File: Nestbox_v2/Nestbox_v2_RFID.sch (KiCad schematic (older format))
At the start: 8 parts, among them J701 RFID_CONN_01X05, Q701 Q_NMOS_DGS

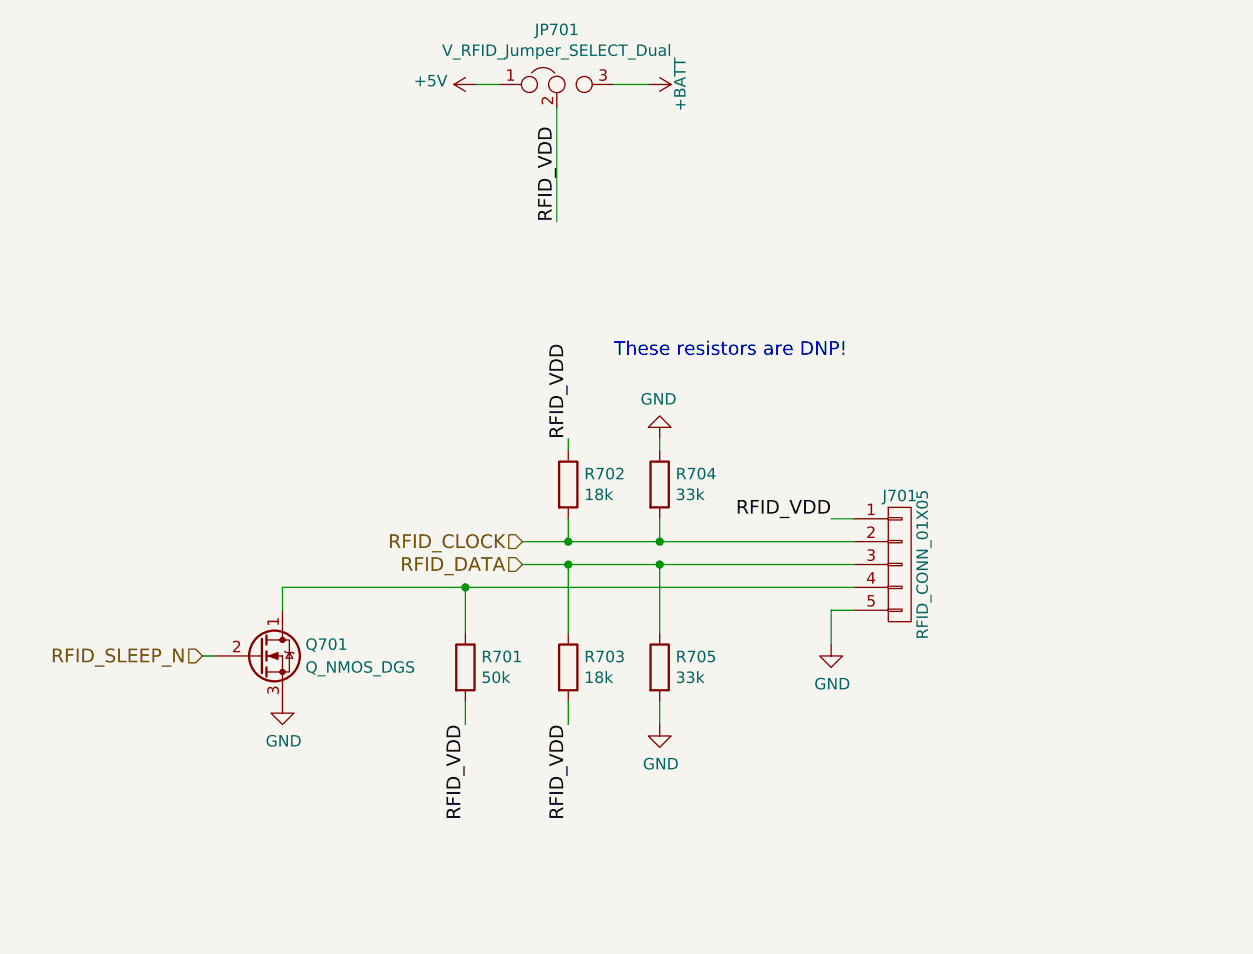
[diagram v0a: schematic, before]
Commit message: finished component placement
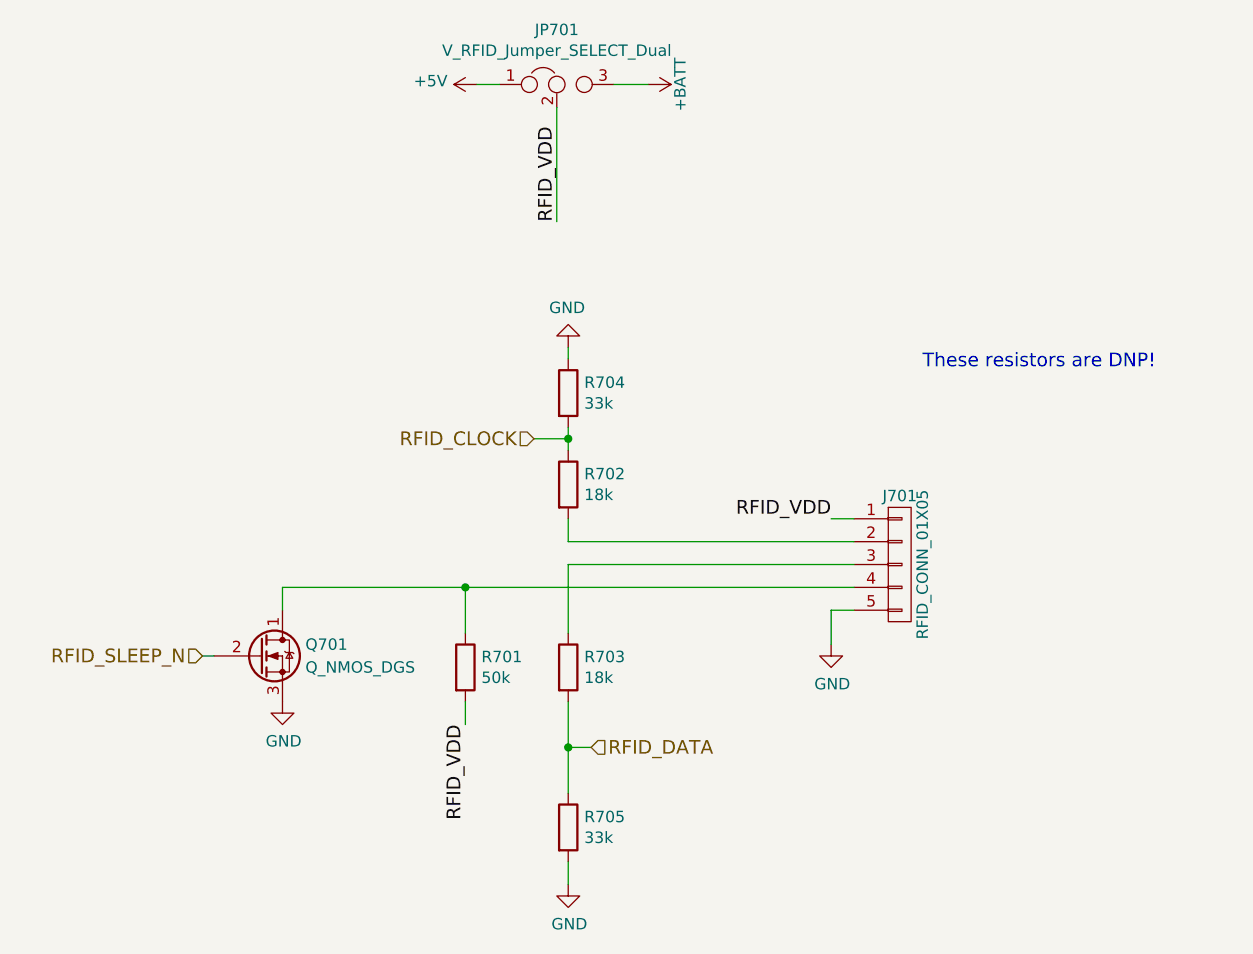
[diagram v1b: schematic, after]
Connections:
- net RFID_CLOCK: now also R702.1; no longer J701.2 (P2), R702.2
- net RFID_DATA: now also R703.2; no longer J701.3 (P3), R703.1
- net RFID_VDD: no longer R702.1, R703.2
- new net: J701.2 (P2), R702.2
- new net: J701.3 (P3), R703.1
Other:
- moved on the sheet: R704, R705
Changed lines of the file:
@@
 RFID_VDD
 $Comp
-L +5V #PWR071
+L +5V #PWR070
 U 1 1 5A0305A8
 P 5200 2300
-F 0 "#PWR071" H 5200 2150 50  0001 C CNN
+F 0 "#PWR070" H 5200 2150 50  0001 C CNN
 F 1 "+5V" V 5215 2428 50  0000 L CNN
 F 2 "" H 5200 2300 50  0001 C CNN
@@
 L R R704
 U 1 1 5AF8AAF5
-P 6000 4050
-F 0 "R704" H 6070 4096 50  0000 L CNN
-F 1 "33k" H 6070 4005 50  0000 L CNN
-F 2 "Resistors_SMD:R_0603" V 5930 4050 50  0001 C CNN
-F 3 "" H 6000 4050 50  0001 C CNN
-	1    6000 4050
+P 5600 3650
+F 0 "R704" H 5670 3696 50  0000 L CNN
+F 1 "33k" H 5670 3605 50  0000 L CNN
+F 2 "Resistors_SMD:R_0603" V 5530 3650 50  0001 C CNN
+F 3 "" H 5600 3650 50  0001 C CNN
+	1    5600 3650
 	1    0    0    -1
 $EndComp
@@
 L R R705
 U 1 1 5AF8AB4E
-P 6000 4850
-F 0 "R705" H 6070 4896 50  0000 L CNN
-F 1 "33k" H 6070 4805 50  0000 L CNN
-F 2 "Resistors_SMD:R_0603" V 5930 4850 50  0001 C CNN
-F 3 "" H 6000 4850 50  0001 C CNN
-	1    6000 4850
-	1    0    0    -1
+P 5600 5550
+F 0 "R705" H 5670 5596 50  0000 L CNN
+F 1 "33k" H 5670 5505 50  0000 L CNN
+F 2 "Resistors_SMD:R_0603" V 5530 5550 50  0001 C CNN
+F 3 "" H 5600 5550 50  0001 C CNN
+	1    5600 5550
+	1    0    0    -1
+$EndComp
+$Comp
+L GND #PWR071
+U 1 1 5AF8ABAA
+P 5600 3450
+F 0 "#PWR071" H 5600 3200 50  0001 C CNN
+F 1 "GND" H 5605 3277 50  0000 C CNN
+F 2 "" H 5600 3450 50  0001 C CNN
+F 3 "" H 5600 3450 50  0001 C CNN
+	1    5600 3450
+	-1   0    0    1
 $EndComp
 $Comp
 L GND #PWR072
-U 1 1 5AF8ABAA
-P 6000 3850
-F 0 "#PWR072" H 6000 3600 50  0001 C CNN
-F 1 "GND" H 6005 3677 50  0000 C CNN
-F 2 "" H 6000 3850 50  0001 C CNN
-F 3 "" H 6000 3850 50  0001 C CNN
-	1    6000 3850
-	-1   0    0    1
+U 1 1 5AF8AC8E
+P 5600 5800
+F 0 "#PWR072" H 5600 5550 50  0001 C CNN
+F 1 "GND" H 5605 5627 50  0000 C CNN
+F 2 "" H 5600 5800 50  0001 C CNN
+F 3 "" H 5600 5800 50  0001 C CNN
+	1    5600 5800
+	1    0    0    -1
 $EndComp
 $Comp
 L GND #PWR073
-U 1 1 5AF8AC8E
-P 6000 5100
-F 0 "#PWR073" H 6000 4850 50  0001 C CNN
-F 1 "GND" H 6005 4927 50  0000 C CNN
-F 2 "" H 6000 5100 50  0001 C CNN
-F 3 "" H 6000 5100 50  0001 C CNN
-	1    6000 5100
-	1    0    0    -1
-$EndComp
-Wire Wire Line
-	6000 5000 6000 5100
-Wire Wire Line
-	6000 3900 6000 3850
-Connection ~ 6000 4400
-Wire Wire Line
-	6000 4400 6000 4700
-Connection ~ 6000 4300
-Wire Wire Line
-	6000 4300 6000 4200
-Wire Wire Line
-	5600 5000 5600 5100
-Wire Wire Line
-	5600 3850 5600 3900
-Connection ~ 5600 4300
-Wire Wire Line
-	5600 4300 5600 4200
-Connection ~ 5600 4400
-Wire Wire Line
-	5600 4400 5600 4700
-Wire Wire Line
-	5400 4400 6850 4400
-Wire Wire Line
-	5400 4300 6850 4300
-Wire Wire Line
-	6750 4200 6850 4200
-Wire Wire Line
-	5550 2400 5550 2900
-Text Label 5600 3850 1    60   ~ 0
-RFID_VDD
-Text Label 5600 5100 3    60   ~ 0
-RFID_VDD
-$Comp
-L GND #PWR074
 U 1 1 5AF8B903
 P 6750 4750
-F 0 "#PWR074" H 6750 4500 50  0001 C CNN
+F 0 "#PWR073" H 6750 4500 50  0001 C CNN
 F 1 "GND" H 6755 4577 50  0000 C CNN
 F 2 "" H 6750 4750 50  0001 C CNN
@@
 	1    0    0    -1
 $EndComp
-Text HLabel 5400 4400 0    60   Input ~ 0
+Text HLabel 5700 5200 2    60   Input ~ 0
 RFID_DATA
-Text HLabel 5400 4300 0    60   Input ~ 0
+Text HLabel 5450 3850 0    60   Input ~ 0
 RFID_CLOCK
-Text Notes 5800 3500 0    60   ~ 0
+Text Notes 7150 3550 0    60   ~ 0
 These resistors are DNP!\n
 $Comp
@@
 Text Label 5150 5100 3    60   ~ 0
 RFID_VDD
-Wire Wire Line
-	5150 5100 5150 5000
-$Comp
-L GND #PWR075
+$Comp
+L GND #PWR074
 U 1 1 5B088780
 P 4350 5000
-F 0 "#PWR075" H 4350 4750 50  0001 C CNN
+F 0 "#PWR074" H 4350 4750 50  0001 C CNN
 F 1 "GND" H 4355 4827 50  0000 C CNN
 F 2 "" H 4350 5000 50  0001 C CNN
@@
 Text HLabel 4000 4800 0    60   Input ~ 0
 RFID_SLEEP_N
-Wire Wire Line
-	4000 4800 4050 4800
-Wire Wire Line
-	4350 4600 4350 4500
-Wire Wire Line
-	4350 4500 6850 4500
 $Comp
 L R R701
@@
 	1    0    0    -1
 $EndComp
-Wire Wire Line
-	5150 4700 5150 4500
-Connection ~ 5150 4500
-Wire Wire Line
-	6750 4600 6850 4600
 $Comp
 L CONN_01X05 J701
@@
 	1    0    0    -1
 $EndComp
-Wire Wire Line
-	6750 4750 6750 4600
-Wire Wire Line
-	5800 2300 5950 2300
-Wire Wire Line
-	5200 2300 5300 2300
-$Comp
-L +BATT #PWR076
+$Comp
+L +BATT #PWR075
 U 1 1 5B08AE2C
 P 5950 2300
-F 0 "#PWR076" H 5950 2150 50  0001 C CNN
+F 0 "#PWR075" H 5950 2150 50  0001 C CNN
 F 1 "+BATT" H 5950 2440 50  0000 C CNN
 F 2 "" H 5950 2300 50  0001 C CNN
@@
 	0    1    1    0
 $EndComp
+Wire Wire Line
+	5600 5700 5600 5800
+Wire Wire Line
+	5600 3500 5600 3450
+Wire Wire Line
+	5600 5000 5600 5400
+Wire Wire Line
+	5600 3800 5600 3900
+Wire Wire Line
+	6750 4200 6850 4200
+Wire Wire Line
+	5550 2400 5550 2900
+Wire Wire Line
+	5150 5100 5150 5000
+Wire Wire Line
+	4000 4800 4050 4800
+Wire Wire Line
+	4350 4600 4350 4500
+Wire Wire Line
+	4350 4500 6850 4500
+Wire Wire Line
+	5150 4700 5150 4500
+Connection ~ 5150 4500
+Wire Wire Line
+	6750 4600 6850 4600
+Wire Wire Line
+	6750 4750 6750 4600
+Wire Wire Line
+	5800 2300 5950 2300
+Wire Wire Line
+	5200 2300 5300 2300
+Wire Wire Line
+	5450 3850 5600 3850
+Connection ~ 5600 3850
+Wire Wire Line
+	5700 5200 5600 5200
+Connection ~ 5600 5200
+Wire Wire Line
+	6850 4300 5600 4300
+Wire Wire Line
+	5600 4300 5600 4200
+Wire Wire Line
+	6850 4400 5600 4400
+Wire Wire Line
+	5600 4400 5600 4700
 $EndSCHEMATC
